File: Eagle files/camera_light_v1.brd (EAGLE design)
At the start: 31.2 x 31.3 mm, 17 parts

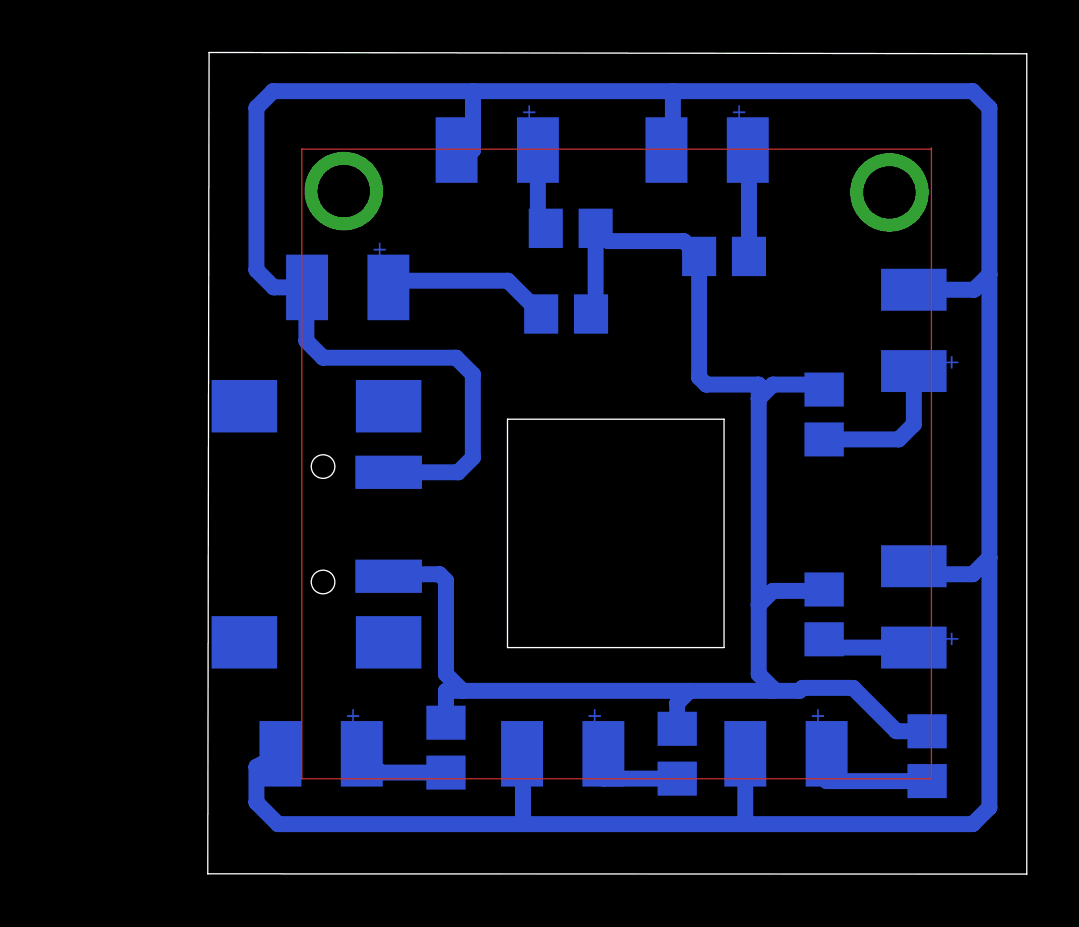
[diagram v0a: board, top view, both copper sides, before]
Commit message: hindi colors added
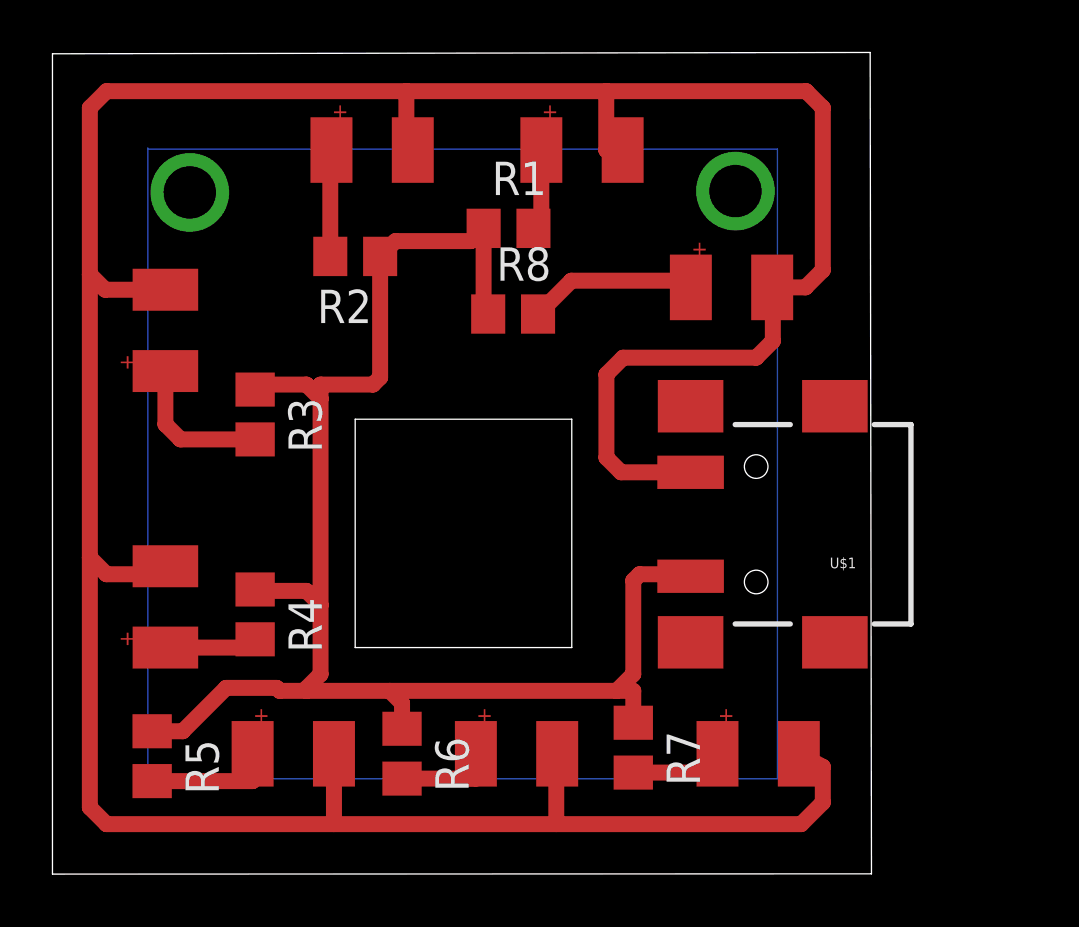
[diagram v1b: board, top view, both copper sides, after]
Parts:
- moved R5 29.5 mm to (-2.07, 4.50), flipped to the top
- moved LED3 27.3 mm to (-0.96, 18.2), flipped to the top
- moved LED4 27.3 mm to (-0.96, 7.63), flipped to the top
- moved LED5 23.9 mm to (0.76, 3.98), flipped to the top
- moved R3 21.7 mm to (1.85, 17.5), flipped to the top
- moved R4 21.7 mm to (1.85, 9.90), flipped to the top
- moved LED2 17.9 mm to (3.77, 27.0), flipped to the top
- moved U$1 16.5 mm to (21.0, 13.3), flipped to the top
- moved R2 14.1 mm to (5.67, 23.5), flipped to the top
- moved LED7 11.6 mm to (18.5, 3.98), flipped to the top
- moved R6 10.5 mm to (7.46, 4.59), flipped to the top
- moved LED8 9.53 mm to (17.5, 21.8), flipped to the top
- moved R7 7.14 mm to (16.3, 4.82), flipped to the top
- moved LED6 6.86 mm to (9.27, 3.98), flipped to the top
- moved R1 2.37 mm to (11.5, 24.6), flipped to the top
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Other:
- outline, holes or cut-outs redrawn
